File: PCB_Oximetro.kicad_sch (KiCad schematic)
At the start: 16 parts, among them J1 USB_A, J2 Conn_01x08, U1 LM1117MP-1.8, U2 MAX30102, U3 LM1117MP-3.3, U5 ESP32-DEVKIT-V1

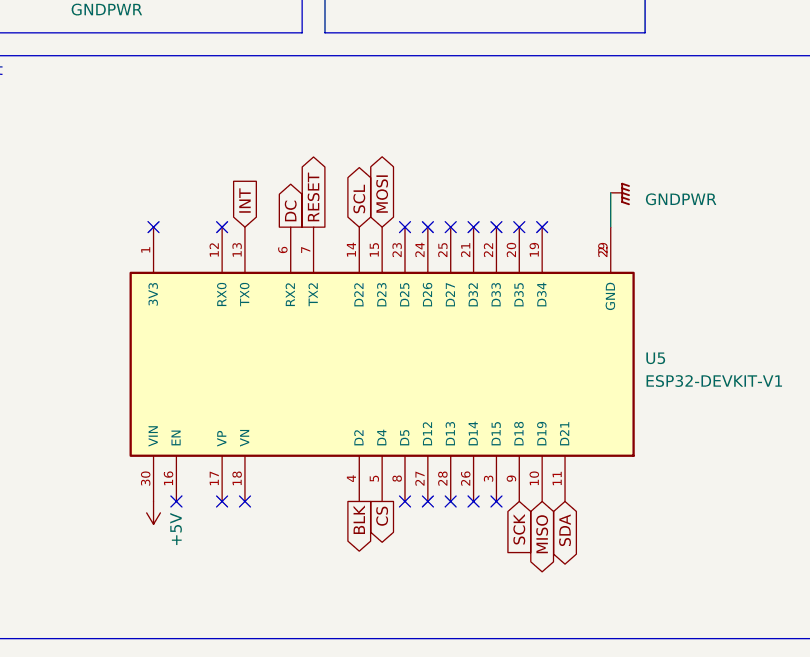
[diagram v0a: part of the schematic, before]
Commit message: 3rd PCB Layout
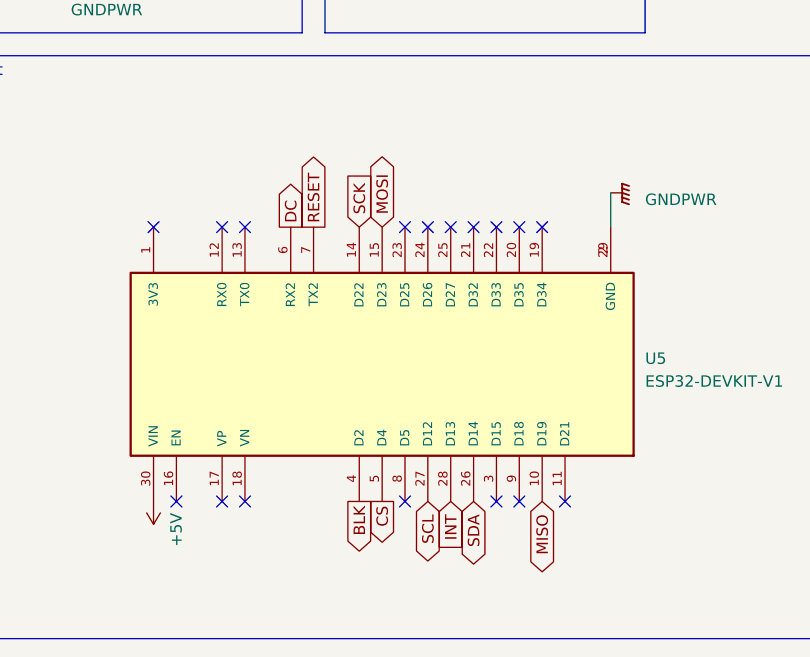
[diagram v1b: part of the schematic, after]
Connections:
- net INT: now also U5.28 (D13); no longer U5.13 (TX0)
- net SCK: now also U5.14 (D22); no longer U5.9 (D18)
- net SCL: now also U5.27 (D12); no longer U5.14 (D22)
- net SDA: now also U5.26 (D14); no longer U5.11 (D21)
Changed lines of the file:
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@@
   (junction (at 135.89 29.21) (diameter 0) (color 0 0 0 0)
   )
-  (no_connect (at 74.93 152.4))
-  (no_connect (at 80.01 152.4))
+  (no_connect (at 85.09 152.4))
+  (no_connect (at 54.61 121.92))
   (no_connect (at 54.61 152.4))
   (no_connect (at 82.55 121.92))
@@
   (no_connect (at 72.39 121.92))
   (no_connect (at 46.99 152.4))
-  (no_connect (at 77.47 152.4))
+  (no_connect (at 90.17 152.4))
   (no_connect (at 77.47 121.92))
   (no_connect (at 80.01 121.92))
@@
     )
   )
-  (global_label "SCL" (shape bidirectional) (at 67.31 121.92 90) (fields_autoplaced)
-    (effects (font (size 1.27 1.27)) (justify left))
-    (property "Intersheetrefs" "${INTERSHEET_REFS}" (at 67.31 114.3953 90)
-      (effects (font (size 1.27 1.27)) (justify left) hide)
+  (global_label "SCL" (shape bidirectional) (at 74.93 152.4 270) (fields_autoplaced)
+    (effects (font (size 1.27 1.27)) (justify right))
+    (property "Intersheetrefs" "${INTERSHEET_REFS}" (at 74.93 159.9247 90)
+      (effects (font (size 1.27 1.27)) (justify right) hide)
     )
   )
@@
     )
   )
-  (global_label "SCK" (shape input) (at 85.09 152.4 270) (fields_autoplaced)
-    (effects (font (size 1.27 1.27)) (justify right))
-    (property "Intersheetrefs" "${INTERSHEET_REFS}" (at 85.09 159.0553 90)
-      (effects (font (size 1.27 1.27)) (justify right) hide)
+  (global_label "SCK" (shape input) (at 67.31 121.92 90) (fields_autoplaced)
+    (effects (font (size 1.27 1.27)) (justify left))
+    (property "Intersheetrefs" "${INTERSHEET_REFS}" (at 67.31 115.2647 90)
+      (effects (font (size 1.27 1.27)) (justify left) hide)
     )
   )
@@
     )
   )
-  (global_label "INT" (shape input) (at 54.61 121.92 90) (fields_autoplaced)
-    (effects (font (size 1.27 1.27)) (justify left))
-    (property "Intersheetrefs" "${INTERSHEET_REFS}" (at 54.61 116.1113 90)
-      (effects (font (size 1.27 1.27)) (justify left) hide)
-    )
-  )
-  (global_label "SDA" (shape bidirectional) (at 90.17 152.4 270) (fields_autoplaced)
-    (effects (font (size 1.27 1.27)) (justify right))
-    (property "Intersheetrefs" "${INTERSHEET_REFS}" (at 90.17 159.9852 90)
-      (effects (font (size 1.27 1.27)) (justify right) hide)
-    )
+  (global_label "INT" (shape input) (at 77.47 152.4 270) (fields_autoplaced)
+    (effects (font (size 1.27 1.27)) (justify right))
+    (property "Intersheetrefs" "${INTERSHEET_REFS}" (at 77.47 158.2087 90)
+      (effects (font (size 1.27 1.27)) (justify right) hide)
+    )
+  )
+  (global_label "SDA" (shape bidirectional) (at 80.01 152.4 270) (fields_autoplaced)
+    (effects (font (size 1.27 1.27)) (justify right))
+    (property "Intersheetrefs" "${INTERSHEET_REFS}" (at 80.01 159.9852 90)
+      (effects (font (size 1.27 1.27)) (justify right) hide)
+    )

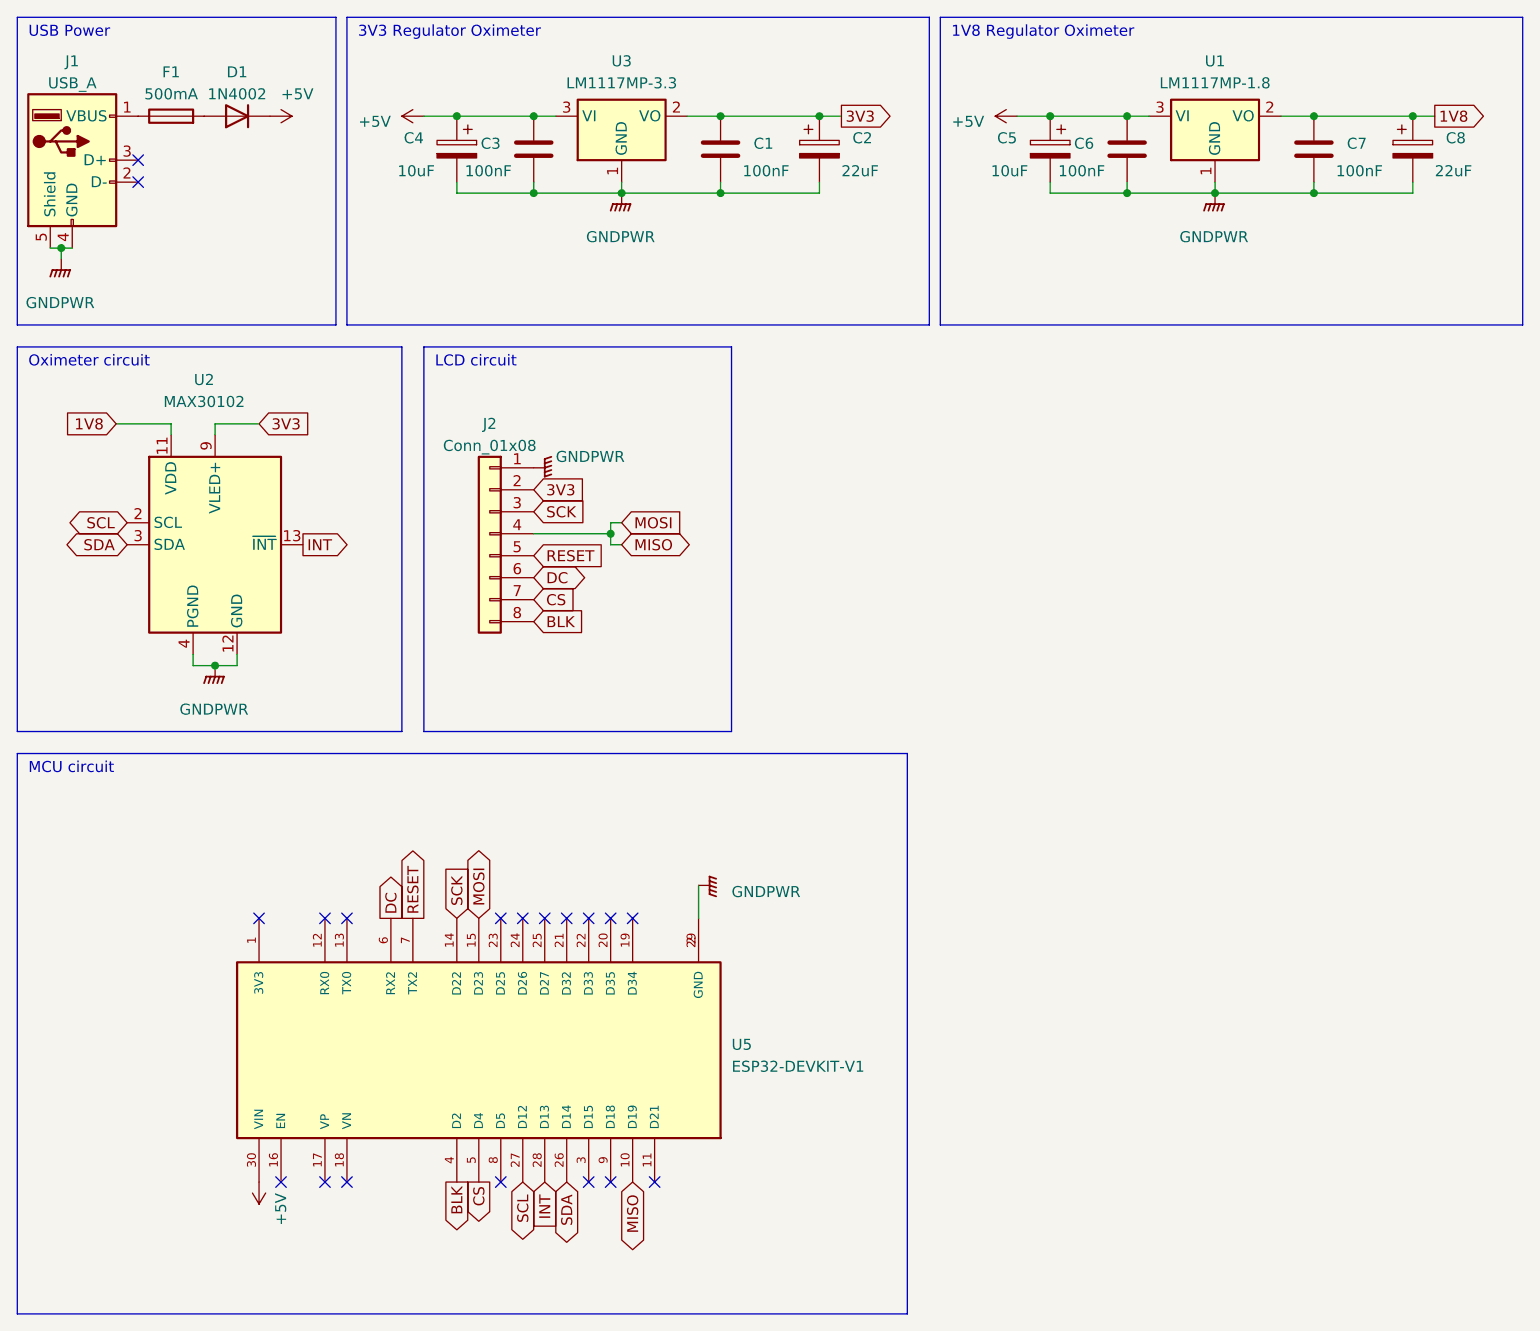
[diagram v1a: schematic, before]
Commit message: 4th PCB Layout
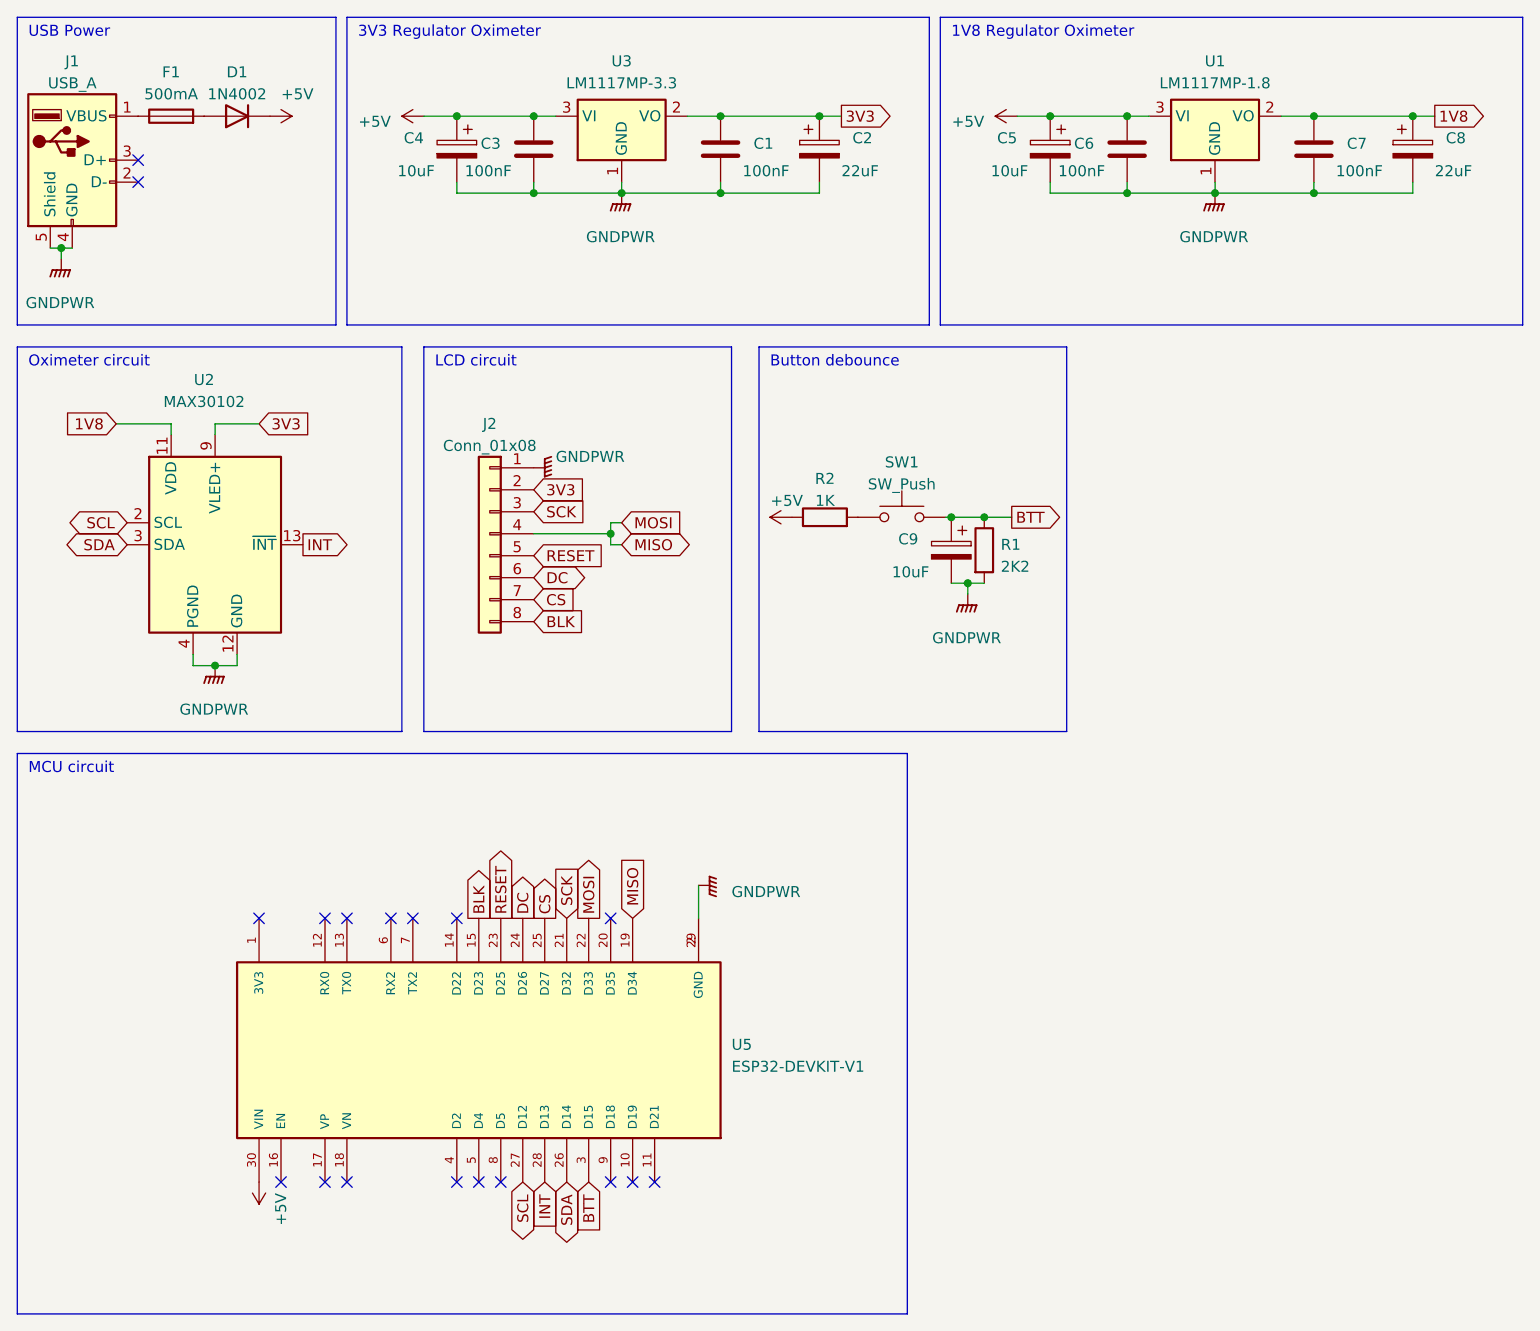
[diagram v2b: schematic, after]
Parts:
- added C9: 10uF, Capacitor_THT:CP_Radial_D5.0mm_P2.50mm, symbol Device:C_Polarized
- added R1: 2K2, Resistor_SMD:R_1206_3216Metric, symbol Device:R
- added R2: 1K, Resistor_SMD:R_1206_3216Metric, symbol Device:R
- added SW1: SW_Push, Button_Switch_THT:SW_Tactile_SPST_Angled_PTS645Vx58-2LFS, symbol Switch:SW_Push
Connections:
- net +5V: now also R2.1
- net BLK: now also U5.15 (D23); no longer U5.4 (D2)
- net CS: now also U5.25 (D27); no longer U5.5 (D4)
- net DC: now also U5.24 (D26); no longer U5.6 (RX2)
- net GNDPWR: now also C9.2, R1.2
- net MISO: now also U5.19 (D34), U5.22 (D33); no longer U5.10 (D19), U5.15 (D23)
- net RESET: now also U5.23 (D25); no longer U5.7 (TX2)
- net SCK: now also U5.21 (D32); no longer U5.14 (D22)
- net BTT: now reaches U5.3 (D15)
- net BTT: now also C9.1, R1.1, SW1.2
- new net: R2.2, SW1.1
- no-connect marks 19 -> 18
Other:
- note added: "Button debounce"
